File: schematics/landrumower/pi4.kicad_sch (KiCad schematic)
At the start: 5 parts, among them J22 IMU, J24 I2C reserve0, J25 I2C reserve1, U2 Raspberry_Pi_2_3

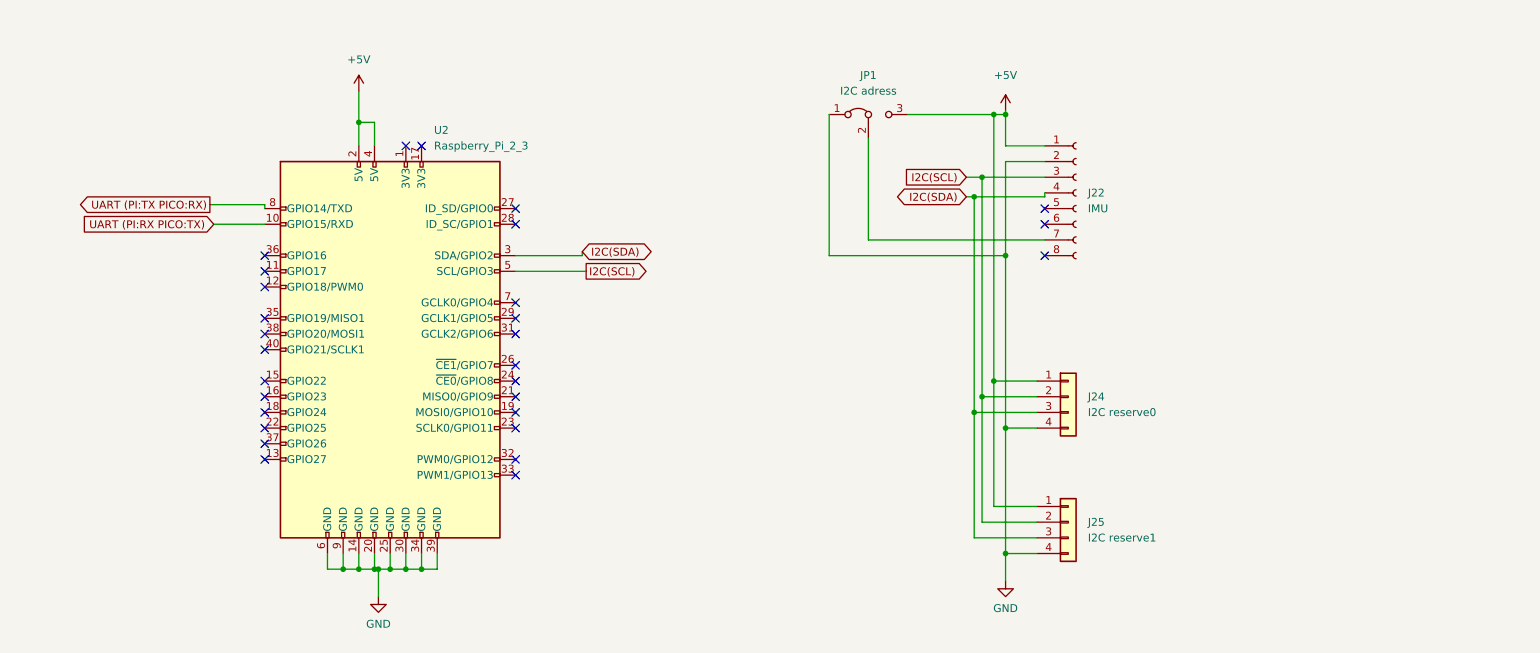
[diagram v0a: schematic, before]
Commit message: PCB changes for Landrumower
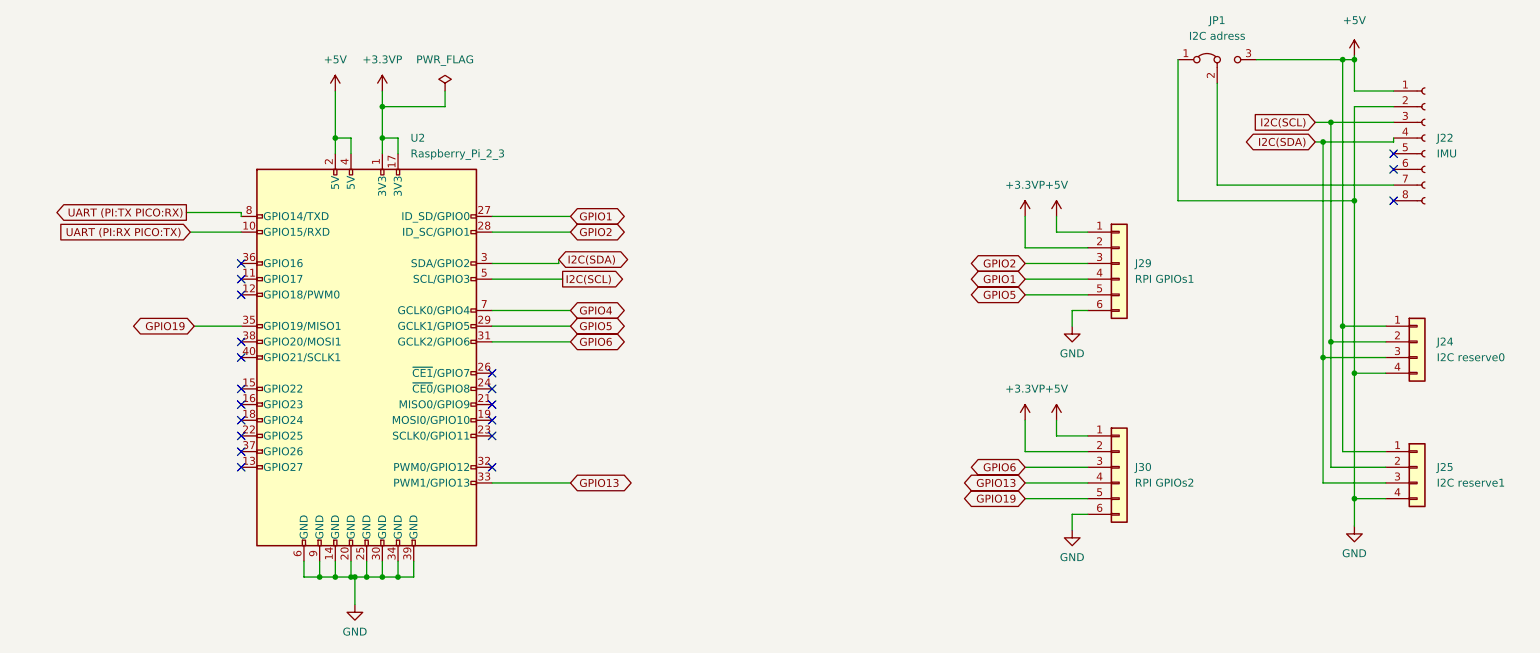
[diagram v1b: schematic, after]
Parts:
- added J29: RPI GPIOs1, Connector_JST:JST_EH_B6B-EH-A_1x06_P2.50mm_Vertical, symbol Connector_Generic:Conn_01x06
- added J30: RPI GPIOs2, Connector_JST:JST_EH_B6B-EH-A_1x06_P2.50mm_Vertical, symbol Connector_Generic:Conn_01x06
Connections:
- net +5V: now also J29.1 (Pin_1), J30.1 (Pin_1)
- net GND: now also J29.6 (Pin_6), J30.6 (Pin_6)
- net +3.3VP: now reaches U2.1 (3V3)
- net +3.3VP: now also U2.17 (3V3), J29.2 (Pin_2), J30.2 (Pin_2)
- net GPIO1: now reaches U2.27 (ID_SD/GPIO0)
- net GPIO1: now also J29.4 (Pin_4)
- net GPIO2: now reaches U2.28 (ID_SC/GPIO1)
- net GPIO2: now also J29.3 (Pin_3)
- net GPIO5: now reaches U2.29 (GCLK1/GPIO5)
- net GPIO5: now also J29.5 (Pin_5)
- net GPIO6: now reaches U2.31 (GCLK2/GPIO6)
- net GPIO6: now also J30.3 (Pin_3)
- net GPIO13: now reaches U2.33 (PWM1/GPIO13)
- net GPIO13: now also J30.4 (Pin_4)
- net GPIO19: now reaches U2.35 (GPIO19/MISO1)
- net GPIO19: now also J30.5 (Pin_5)
- net GPIO4: now reaches U2.7 (GCLK0/GPIO4)
- no-connect marks 29 -> 20
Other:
- moved on the sheet: J22, J24, J25, JP1, U2
